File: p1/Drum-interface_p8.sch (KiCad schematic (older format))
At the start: 91 parts, among them P1 CONN-02x05, U1 CD4001, U2 082, U3 082, U4 NJM, U5 082, U6 082

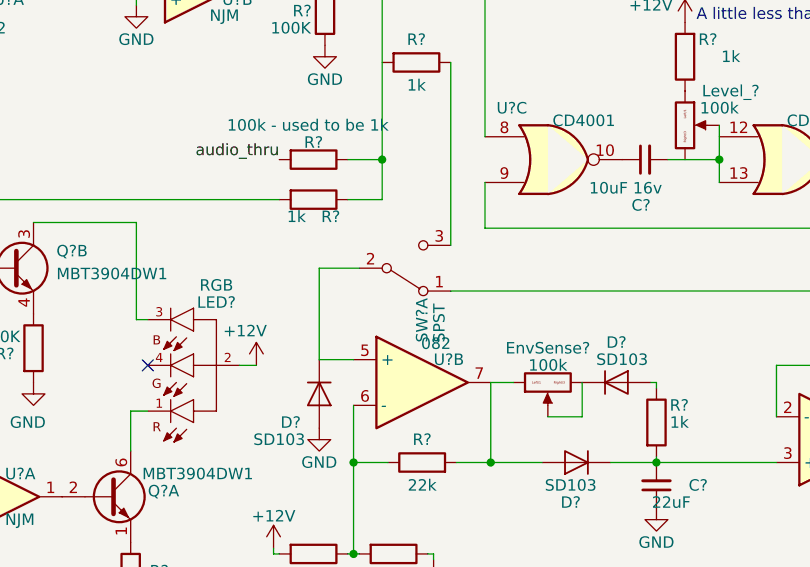
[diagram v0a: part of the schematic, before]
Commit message: setup power
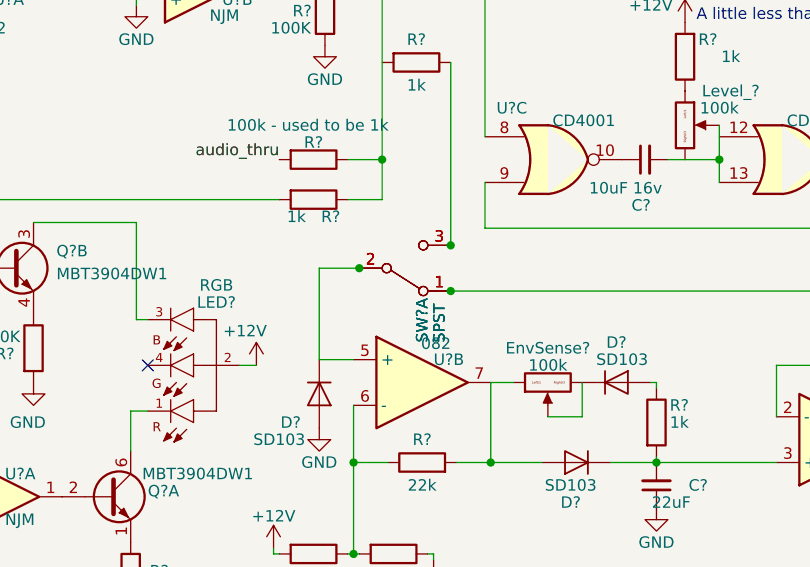
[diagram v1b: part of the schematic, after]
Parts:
- added SW?: SPST, 4ms_Switch:Slide_Switch_Runrun_SS22D06, symbol 4ms-mech:DPDT-shielded-sep
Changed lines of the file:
@@
 Wire Wire Line
 	5125 1925 5125 2725
+$Comp
+L 4ms-mech:DPDT-shielded-sep SW?
+U 1 1 5DEE278C
+P 5225 3200
+F 0 "SW?" V 5300 3525 50  0000 R CNN
+F 1 "SPST" V 5375 3525 50  0000 R CNN
+F 2 "4ms_Switch:Slide_Switch_Runrun_SS22D06" H 5225 3200 50  0001 C CNN
+F 3 "" H 5225 3200 50  0001 C CNN
+F 4 "Mouser" H -325 -225 50  0001 C CNN "Manufacturer"
+F 5 "Substitution OK" H -325 -225 50  0001 C CNN "Comments"
+	1    5225 3200
+	1    0    0    1
+$EndComp
+Connection ~ 5425 3300
+Connection ~ 5025 3200
+Connection ~ 5425 3100
 $EndSCHEMATC
